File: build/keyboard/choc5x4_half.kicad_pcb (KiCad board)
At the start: 2 copper layers, 103.2 x 92.2 mm, 40 parts, among them SW1 Kailh Choc V1 / V2, SW10 Kailh Choc V1 / V2, SW11 Kailh Choc V1 / V2, SW12 Kailh Choc V1 / V2, SW13 Kailh Choc V1 / V2, SW14 Kailh Choc V1 / V2, SW15 Kailh Choc V1 / V2, SW16 Kailh Choc V1 / V2, SW17 Kailh Choc V1 / V2, SW18 Kailh Choc V1 / V2, SW19 Kailh Choc V1 / V2, SW2 Kailh Choc V1 / V2, SW20 Kailh Choc V1 / V2, SW3 Kailh Choc V1 / V2, SW4 Kailh Choc V1 / V2, SW5 Kailh Choc V1 / V2, SW6 Kailh Choc V1 / V2, SW7 Kailh Choc V1 / V2, SW8 Kailh Choc V1 / V2, SW9 Kailh Choc V1 / V2

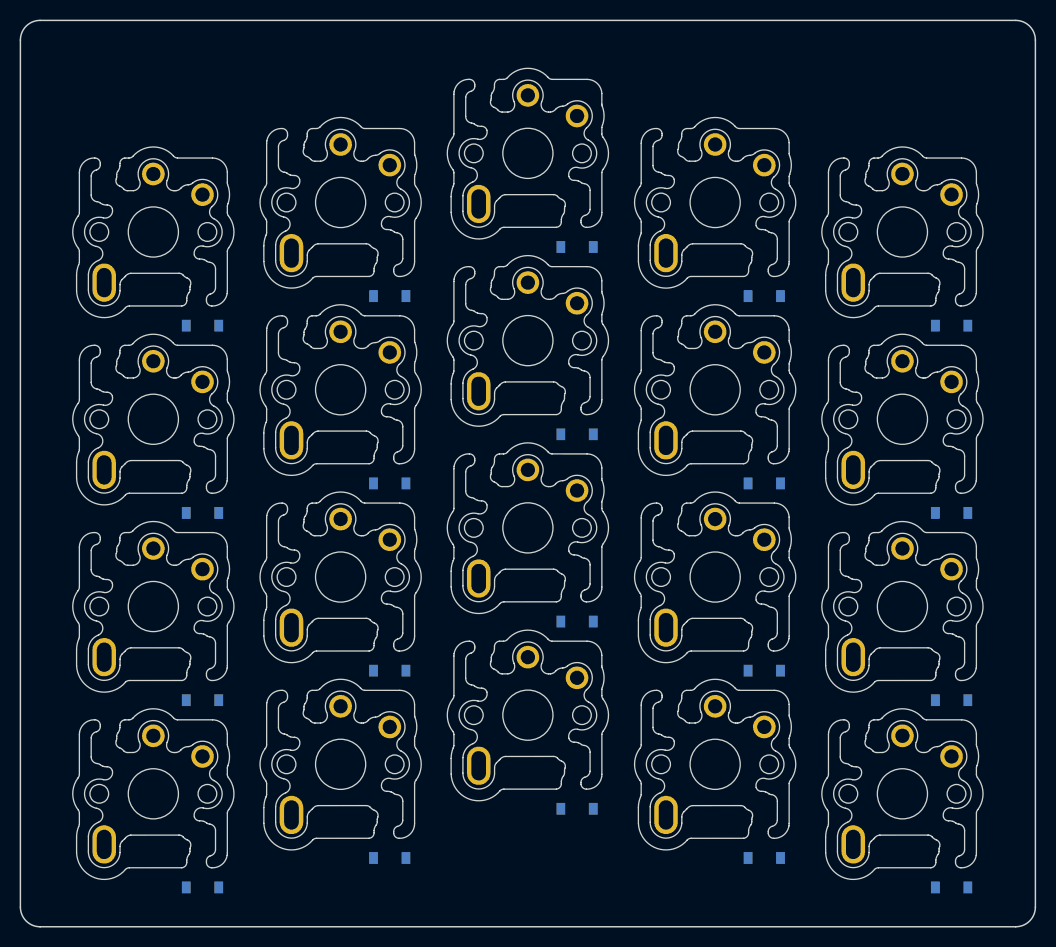
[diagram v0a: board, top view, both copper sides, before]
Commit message: update
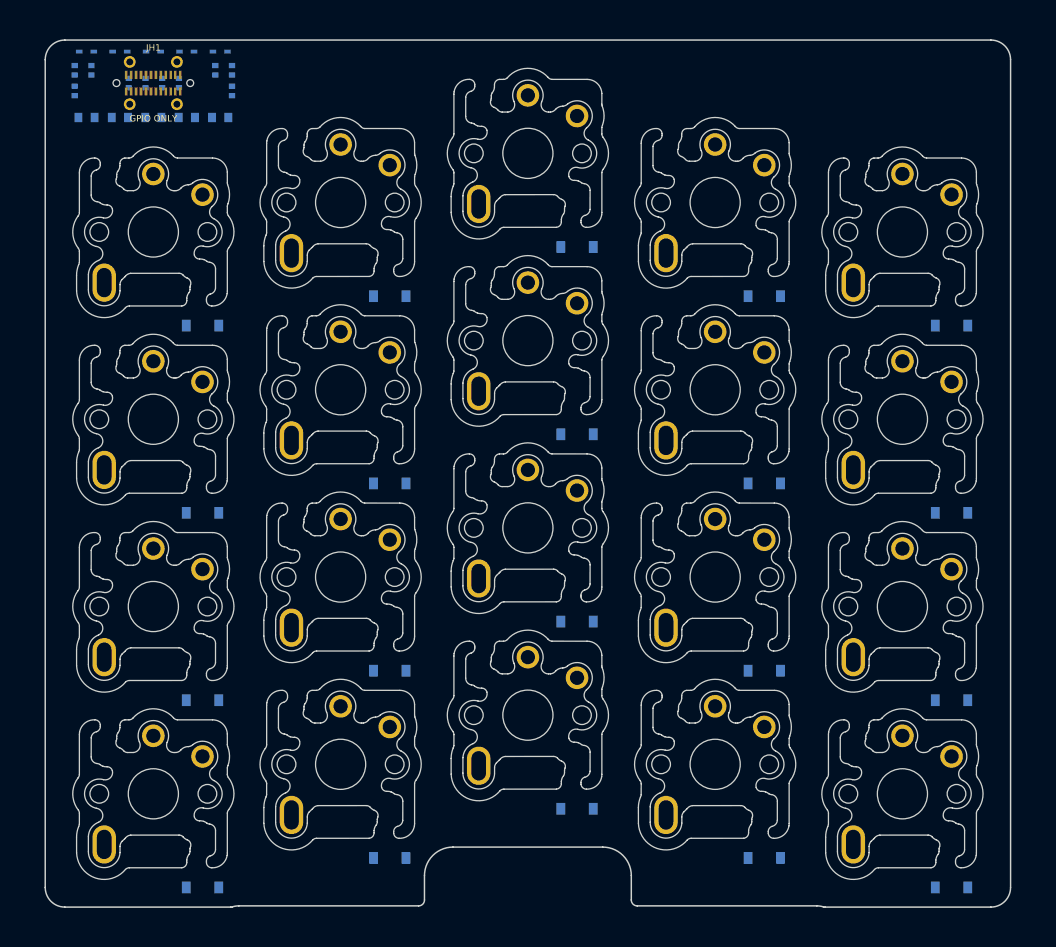
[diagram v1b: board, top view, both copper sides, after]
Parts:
- added EH1: TPD1E05U06DYA, keyboard-design:sod523, B.Cu at (53.2, 44.5)
- added EH2: TPD1E05U06DYA, keyboard-design:sod523, B.Cu at (56.6, 44.5)
- added EH3: TPD1E05U06DYA, keyboard-design:sod523, B.Cu at (60.0, 44.5)
- added EH4: TPD1E05U06DYA, keyboard-design:sod523, B.Cu at (63.4, 44.5)
- added EH5: TPD1E05U06DYA, keyboard-design:sod523, B.Cu at (66.8, 44.5)
- added JH1: USB4115-03-C / GPIO ONLY, keyboard-design:usb4115, F.Cu at (60.0, 47.7)
- added RCH1: 1k contact isolation, keyboard-design:r0402, B.Cu at (52.0, 46.4)
- added RCH10: 1k contact isolation, keyboard-design:r0402, B.Cu at (68.0, 48.5)
- added RCH2: 1k contact isolation, keyboard-design:r0402, B.Cu at (53.7, 46.4)
- added RCH3: 1k contact isolation, keyboard-design:r0402, B.Cu at (52.0, 48.5)
- added RCH4: 1k contact isolation, keyboard-design:r0402, B.Cu at (57.5, 47.7)
- added RCH5: 1k contact isolation, keyboard-design:r0402, B.Cu at (59.2, 47.7)
- added RCH6: 1k contact isolation, keyboard-design:r0402, B.Cu at (60.9, 47.7)
- added RCH7: 1k contact isolation, keyboard-design:r0402, B.Cu at (62.6, 47.7)
- added RCH8: 1k contact isolation, keyboard-design:r0402, B.Cu at (66.3, 46.4)
- added RCH9: 1k contact isolation, keyboard-design:r0402, B.Cu at (68.0, 46.4)
- added RH1: 1k, keyboard-design:r0603, B.Cu at (53.2, 51.2)
- added RH2: 1k, keyboard-design:r0603, B.Cu at (56.6, 51.2)
- added RH3: 1k, keyboard-design:r0603, B.Cu at (60.0, 51.2)
- added RH4: 1k, keyboard-design:r0603, B.Cu at (63.4, 51.2)
- added RH5: 1k, keyboard-design:r0603, B.Cu at (66.8, 51.2)
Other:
- board size 103.2 x 92.2 mm -> 98.2 x 88.2 mm
